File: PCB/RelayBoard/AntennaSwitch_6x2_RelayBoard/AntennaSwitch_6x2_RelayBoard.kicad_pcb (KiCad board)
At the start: 2 copper layers, 200 x 105 mm, 36 parts, among them J1 Conn_Coaxial, J2 Conn_Coaxial, J3 Conn_Coaxial, J4 Conn_Coaxial, J5 Conn_Coaxial, J6 Conn_Coaxial, J7 Conn_Coaxial, J8 Conn_Coaxial, K1 FINDER-40.61, K10 FINDER-40.61, K11 FINDER-40.61, K12 FINDER-40.61, K13 FINDER-40.61, K14 FINDER-40.61, K15 FINDER-40.61, K16 FINDER-40.61, K17 FINDER-40.61, K18 FINDER-40.61, K2 FINDER-40.61, K3 FINDER-40.61, K4 FINDER-40.61, K5 FINDER-40.61, K6 FINDER-40.61, K7 FINDER-40.61, K8 FINDER-40.61, K9 FINDER-40.61, U1 ULN2003, U2 ULN2003, U3 74HC04, U4 74HC04

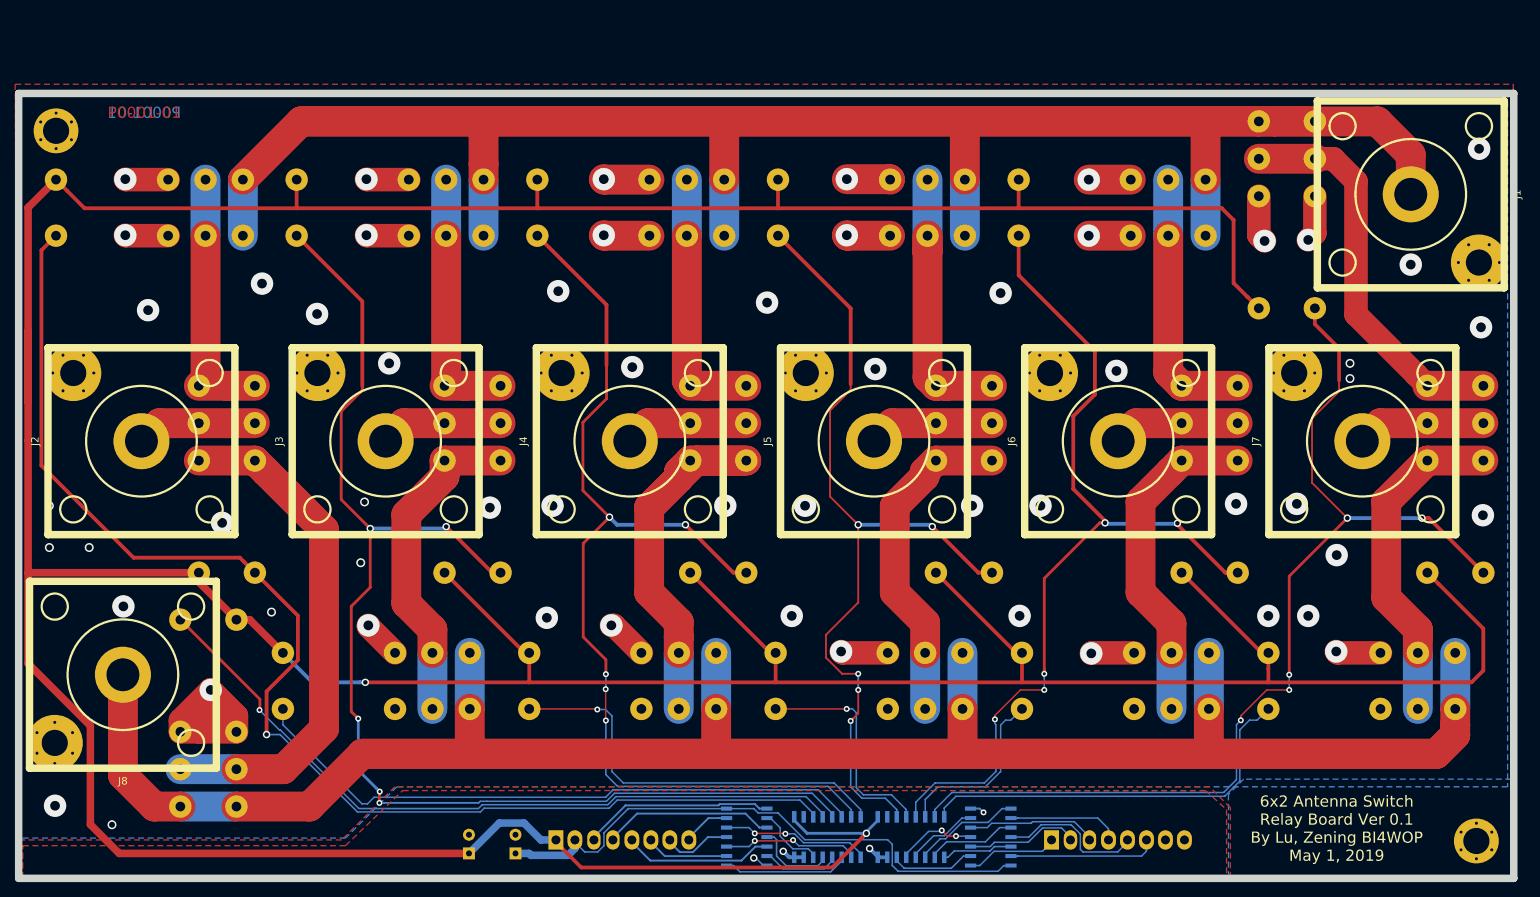
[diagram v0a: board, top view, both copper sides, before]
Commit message: FS Tools
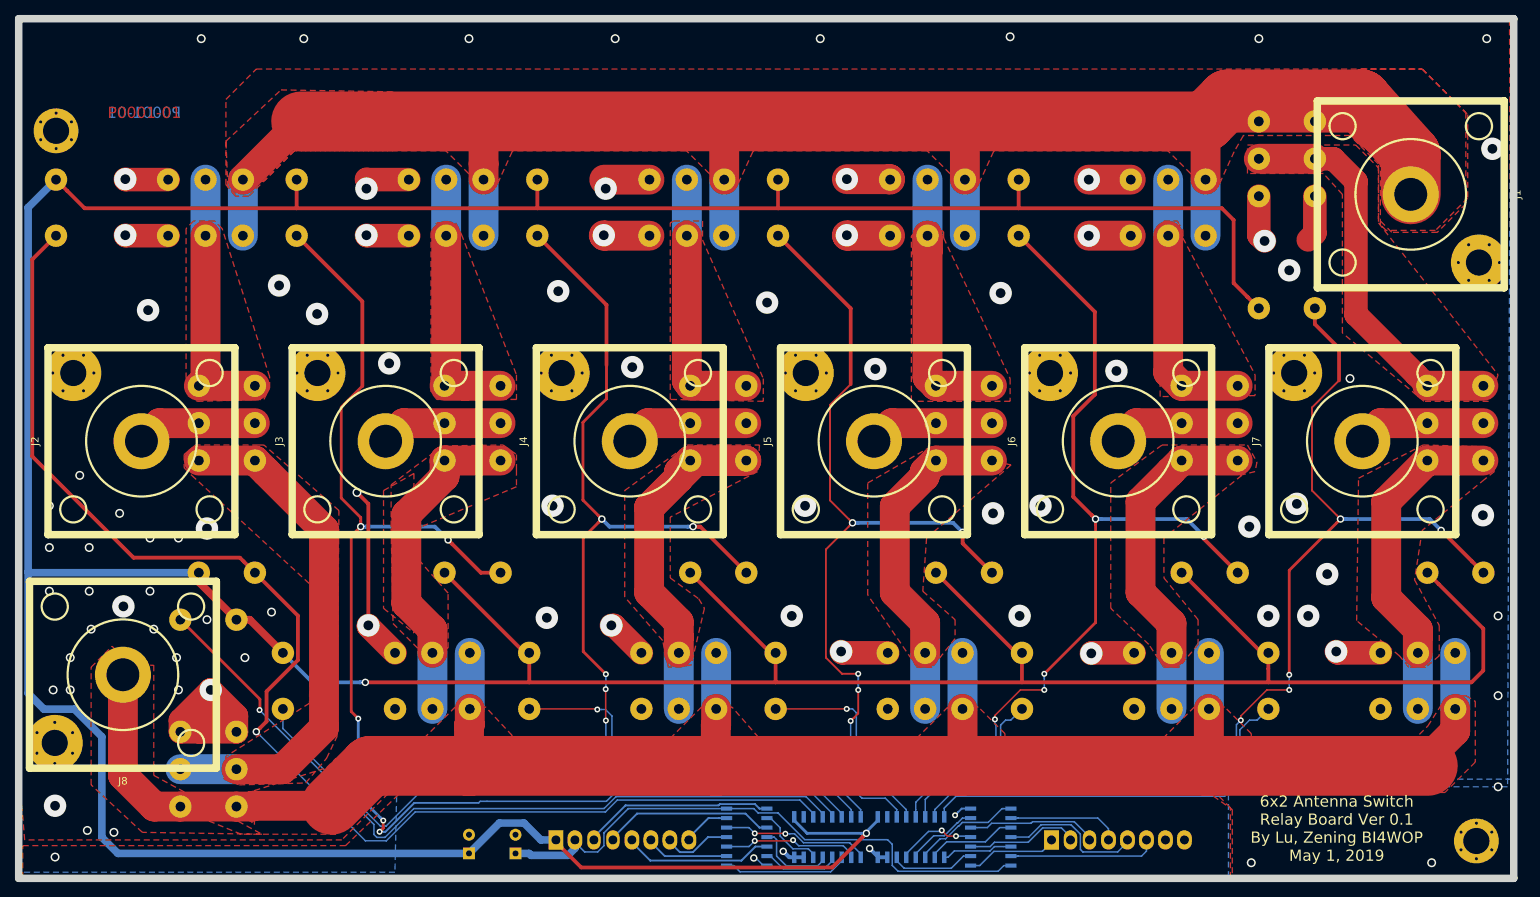
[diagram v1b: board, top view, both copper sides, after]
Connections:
- REF** pad 1: A -> GNDPWR
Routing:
- net B: track 409.6 -> 272.4 mm
- net A: track 533.8 -> 582.2 mm
- net GNDPWR: track 133.7 -> 152.1 mm, vias 84 -> 101
- net +12V: track 712.1 -> 705.1 mm
- net Net-(K1-PadA1): track 171.1 -> 177.0 mm
- net Net-(K2-PadA1): track 168.4 -> 173.7 mm
- net Net-(K13-PadA1): track 99.4 -> 103.4 mm
- net Net-(K14-PadA1): track 83.8 -> 86.6 mm
- net Net-(K10-PadA1): track 114.7 -> 115.8 mm
- net GND: track 12.7 -> 13.2 mm, vias 4 -> 5
- added copper zone on F.Cu, net A
- added copper zone on F.Cu, net B
- added copper zone on F.Cu, net Net-(K1-Pad11)
- added copper zone on F.Cu, net Net-(K10-Pad12)
- added copper zone on F.Cu, net Net-(K10-Pad14)
- added copper zone on F.Cu, net Net-(K11-Pad12)
- added copper zone on F.Cu, net Net-(K11-Pad14)
- added copper zone on F.Cu, net Net-(K12-Pad12)
- added copper zone on F.Cu, net Net-(K12-Pad14)
- added copper zone on F.Cu, net Net-(K13-Pad11)
- added copper zone on F.Cu, net Net-(K14-Pad11)
- added copper zone on F.Cu, net Net-(K15-Pad11)
- added copper zone on F.Cu, net Net-(K2-Pad11)
- added copper zone on F.Cu, net Net-(K3-Pad11)
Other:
- board size 200 x 105 mm -> 200 x 115 mm
- net class RF: clearance 2 -> 1.5
